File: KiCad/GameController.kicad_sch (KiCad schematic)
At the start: 14 parts, among them SW1 SW_Push, SW10 SW_Push, SW2 SW_Push, SW3 SW_Push, SW4 SW_Push, SW5 SW_Push, SW6 SW_Push, SW7 SW_Push, SW8 SW_Push, SW9 SW_Push, U1 COM-09032, U2 COM-09032, U3 MCP3008

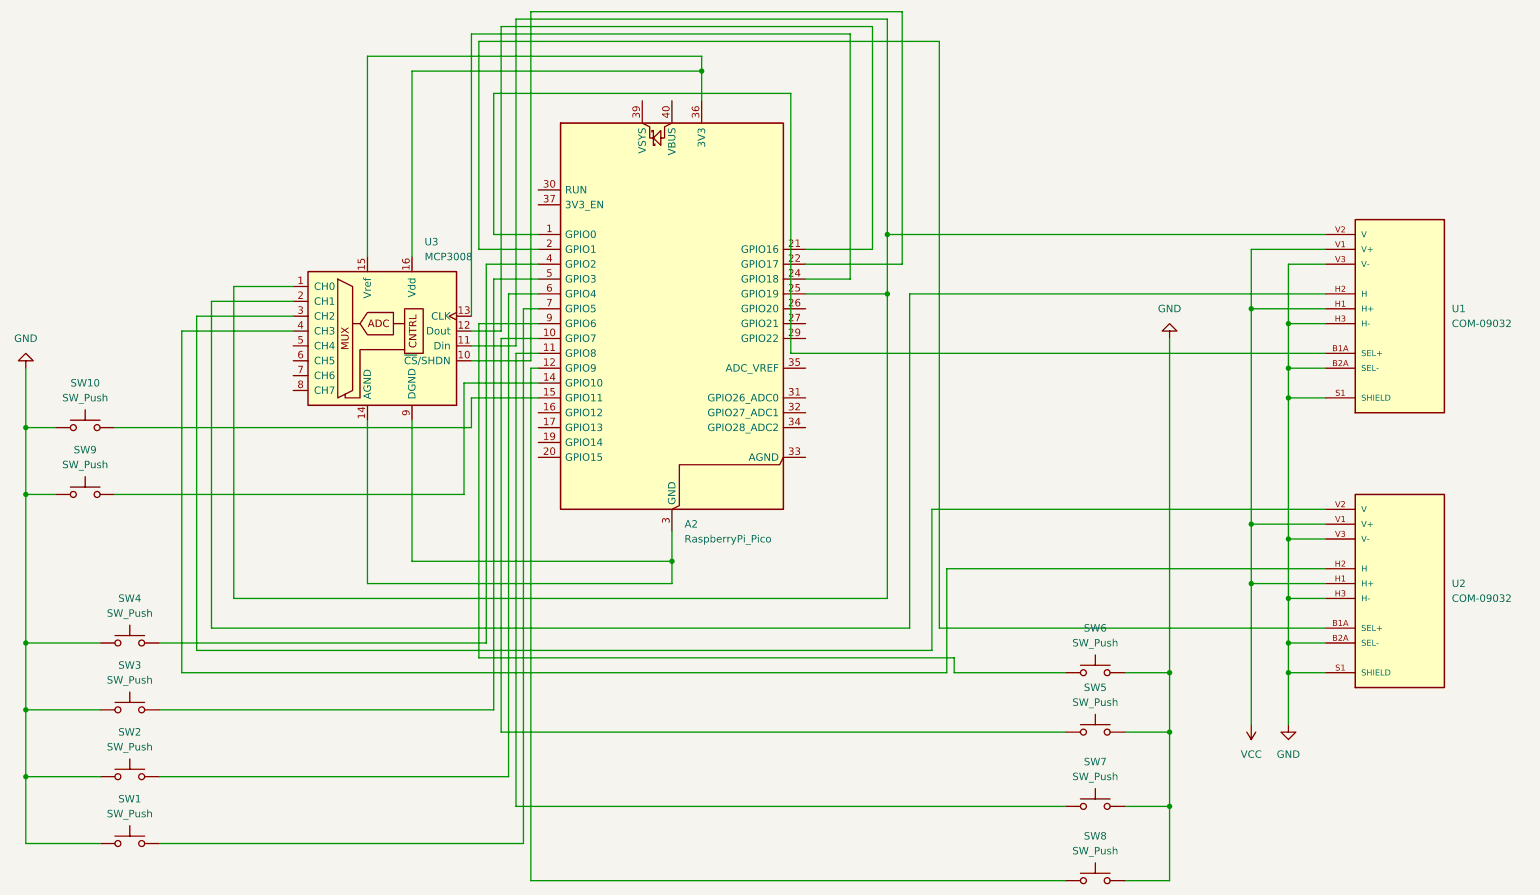
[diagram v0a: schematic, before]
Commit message: UP
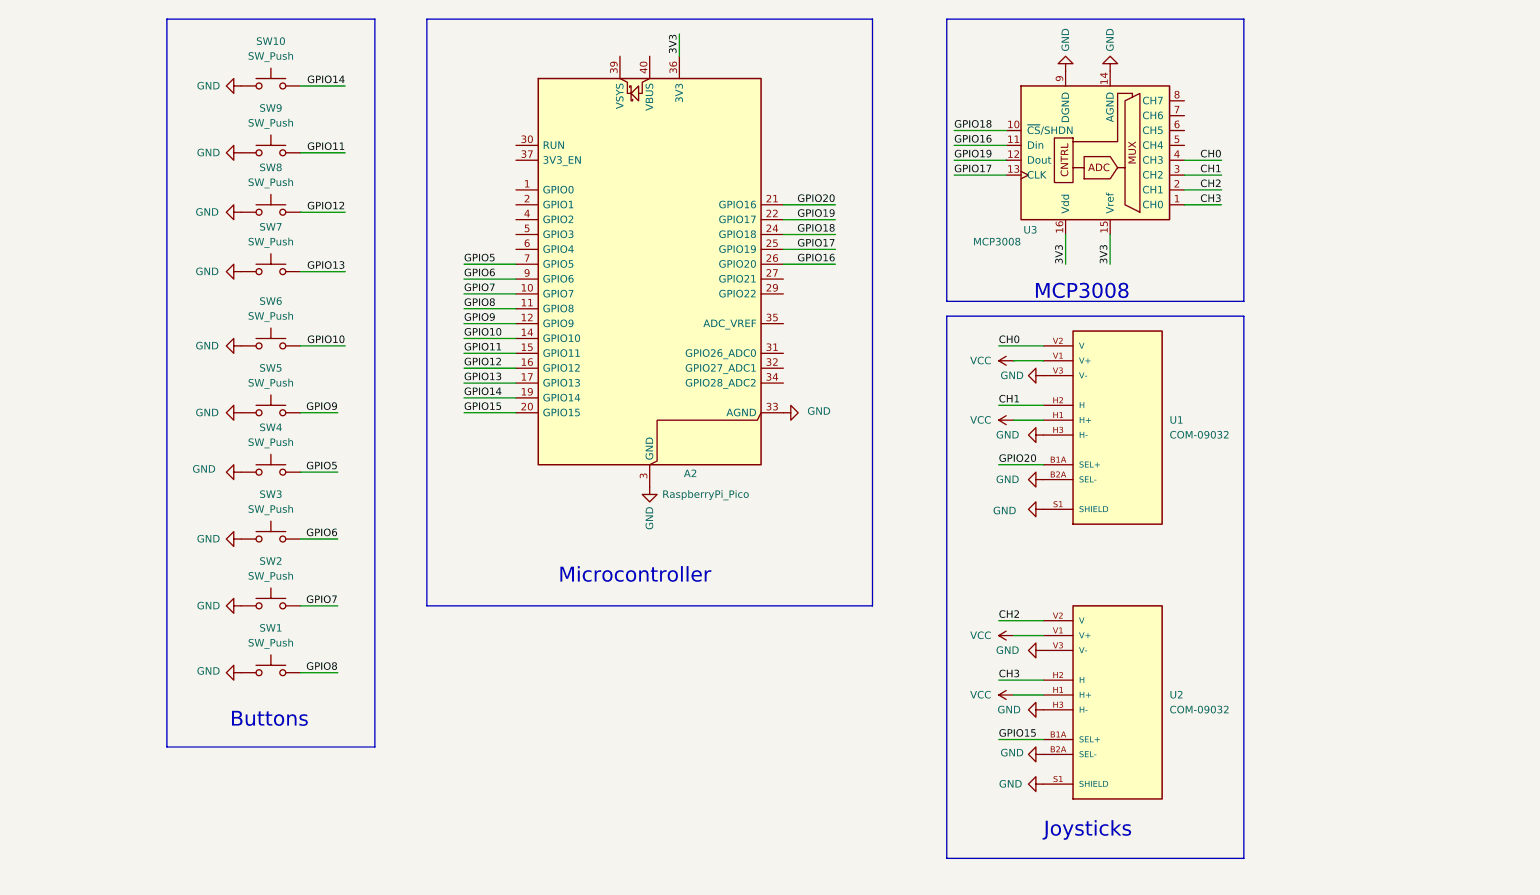
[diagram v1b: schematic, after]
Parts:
- A2: footprint Module:RaspberryPi_Pico_Common_Unspecified -> Module:RaspberryPi_Pico_Common_THT
- renumbered SW8 to SW5, SW7 to SW6, SW5 to SW7, SW6 to SW8
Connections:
- net GND: now also A2.13 (GND), A2.18 (GND), A2.23 (GND), A2.28 (GND), A2.3 (GND), A2.33 (AGND), A2.38 (GND), A2.8 (GND), SW5.1, SW6.1, SW7.1, SW8.1, U3.14 (AGND), U3.9 (DGND); no longer SW5.2, SW6.2, SW7.2, SW8.2
- net GPIO5: now reaches A2.7 (GPIO5)
- net GPIO5: now also SW4.2; no longer SW1.2
- net GPIO18: now reaches U3.10 (~{CS}/SHDN)
- net GPIO18: now also A2.24 (GPIO18); no longer A2.22 (GPIO17)
- net GPIO19: now reaches U3.12 (Dout)
- net GPIO19: now also A2.22 (GPIO17); no longer A2.21 (GPIO16)
- net GPIO17: now reaches U3.13 (CLK)
- net GPIO17: now also A2.25 (GPIO19); no longer A2.24 (GPIO18)
- net 3V3: now reaches A2.36 (3V3), U3.15 (Vref), U3.16 (Vdd)
- net CH1: now reaches U1.H2 (H)
- net CH1: now also U3.3 (CH2); no longer U3.2 (CH1)
- net CH2: now reaches U2.V2 (V)
- net CH2: now also U3.2 (CH1); no longer U3.3 (CH2)
- net CH0: now reaches U3.4 (CH3)
- net CH0: now also U1.V2 (V); no longer U2.H2 (H)
- net GPIO6: now reaches A2.9 (GPIO6)
- net GPIO6: now also SW3.2; no longer SW8.1
- net at A2.4 (GPIO2): no longer SW4.2
- net GPIO9: now reaches A2.12 (GPIO9)
- net GPIO9: now also SW5.2; no longer SW5.1
- net at A2.6 (GPIO4): no longer SW2.2
- net GPIO7: now reaches A2.10 (GPIO7)
- net GPIO7: now also SW2.2; no longer SW7.1
- net GPIO8: now reaches A2.11 (GPIO8)
- net GPIO8: now also SW1.2; no longer SW6.1
- net GPIO11: now reaches A2.15 (GPIO11)
- net GPIO11: now also SW9.2; no longer SW10.2
- net at A2.1 (GPIO0): no longer U1.B1A (SEL+)
- net GPIO10: now reaches A2.14 (GPIO10)
- net GPIO10: now also SW6.2; no longer SW9.2
- net GPIO12: now reaches A2.16 (GPIO12)
- net GPIO12: now also SW8.2
- net GPIO13: now reaches A2.17 (GPIO13)
- net GPIO13: now also SW7.2
- net GPIO14: now reaches A2.19 (GPIO14)
- net GPIO14: now also SW10.2
- net at A2.2 (GPIO1): no longer U2.B1A (SEL+)
- net GPIO15: now reaches A2.20 (GPIO15)
- net GPIO15: now also U2.B1A (SEL+)
- net GPIO16: now reaches A2.26 (GPIO20)
- net GPIO16: now also U3.11 (Din)
- net at A2.5 (GPIO3): no longer SW3.2
- new net CH3: U2.H2 (H), U3.1 (CH0)
- new net GPIO20: A2.21 (GPIO16), U1.B1A (SEL+)
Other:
- note added: "Buttons"
- note added: "Joysticks"
- note added: "MCP3008"
- note added: "Microcontroller"
- moved on the sheet: A2, SW1, SW10, SW2, SW3, SW4, SW5, SW6, SW7, SW8, SW9, U1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
